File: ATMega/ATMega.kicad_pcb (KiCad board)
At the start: 2 copper layers, 7 parts

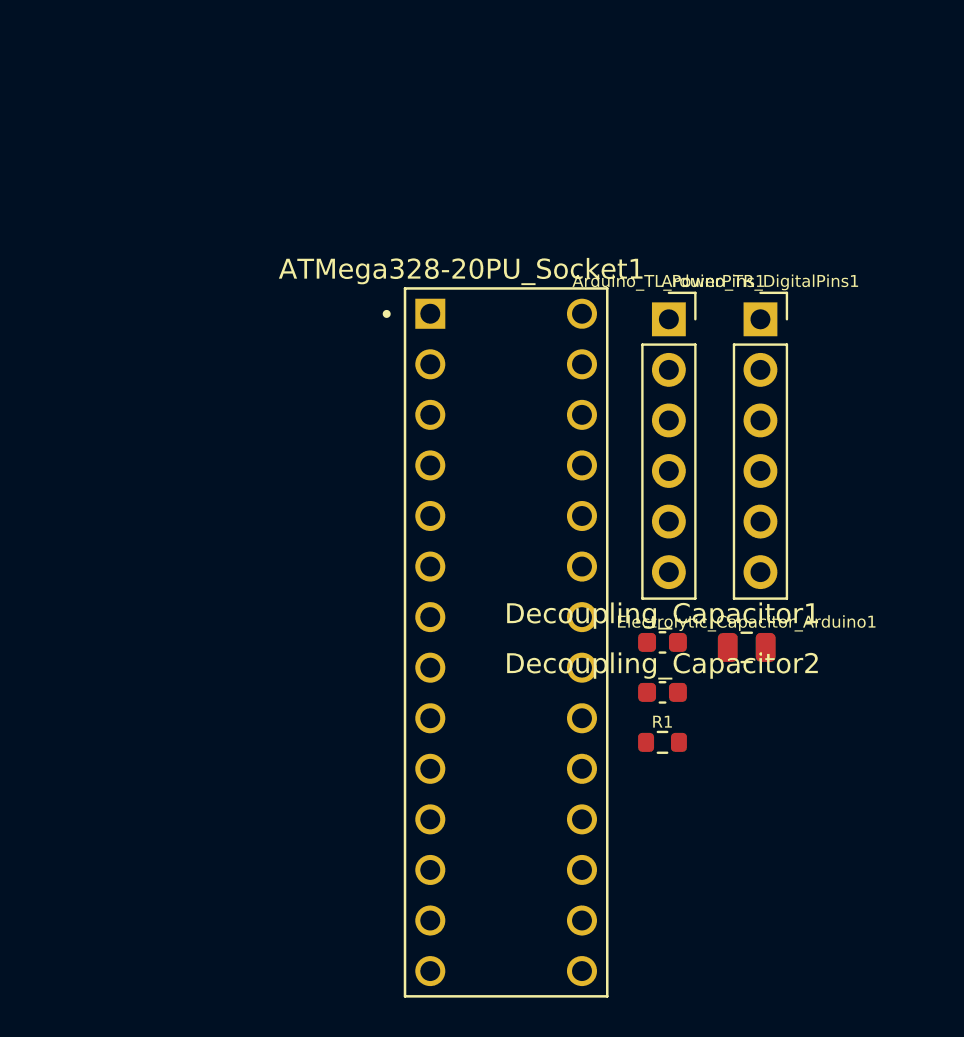
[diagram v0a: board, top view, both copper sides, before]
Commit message: ATMega adjust
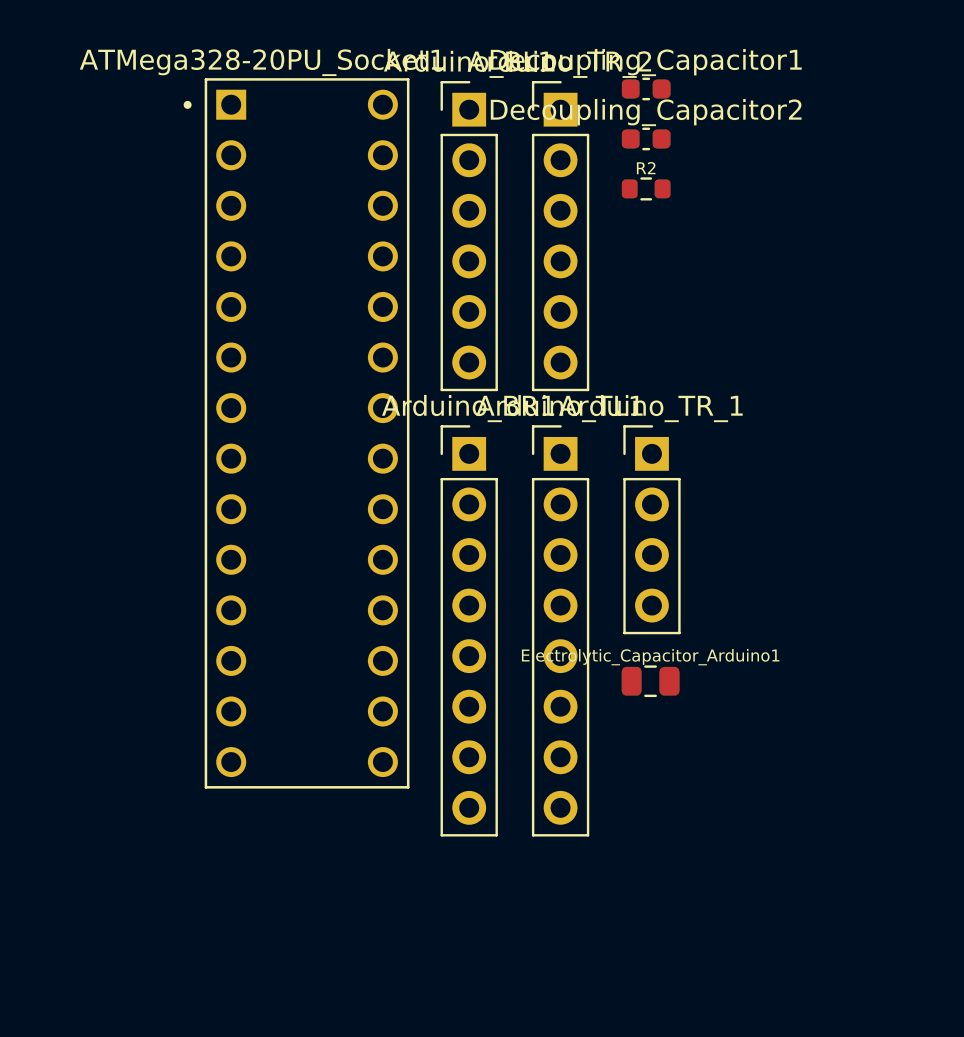
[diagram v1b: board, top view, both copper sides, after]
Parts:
- removed Arduino_TL_PowerPins1, Arduino_TR_DigitalPins1: Conn_01x06_Female, rsx_headers:PinSocket_1x06_P2.54mm_Vertical
- removed R1: 10k, rsx_resistors:R_0603_1608Metric
- added Arduino_BL1: header_1x6_arduino, Connector_PinHeader_2.54mm:PinHeader_1x06_P2.54mm_Vertical, F.Cu at (28.8, 17.3)
- added Arduino_BR1: header_1x8_arduino, Connector_PinHeader_2.54mm:PinHeader_1x08_P2.54mm_Vertical, F.Cu at (28.8, 34.6)
- added Arduino_TL1: header_1x8_arduino, Connector_PinHeader_2.54mm:PinHeader_1x08_P2.54mm_Vertical, F.Cu at (33.4, 34.6)
- added Arduino_TR_1: header_1x4_arduino, Connector_PinHeader_2.54mm:PinHeader_1x04_P2.54mm_Vertical, F.Cu at (38.0, 34.6)
- added Arduino_TR_2: header_1x6_arduino, Connector_PinHeader_2.54mm:PinHeader_1x06_P2.54mm_Vertical, F.Cu at (33.4, 17.3)
- added R2: 10k, rsx_resistors:R_0603_1608Metric, F.Cu at (37.7, 21.3)
- moved Decoupling_Capacitor1 27.8 mm to (37.7, 16.3)
- moved Decoupling_Capacitor2 27.8 mm to (37.7, 18.8)
- moved ATMega328-20PU_Socket1 14.5 mm to (20.7, 33.6)
- moved Electrolytic_Capacitor_Arduino1 5.12 mm to (38.0, 46.0)
